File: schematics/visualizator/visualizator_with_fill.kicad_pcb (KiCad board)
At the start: 2 copper layers, 39.3 x 43.2 mm, 20 parts, among them J1 5V, J2 WS2812, J3 Audio, SW1 COLOR, SW2 PATTERN, U1 ATmega328-16PU, Y1 16MHz

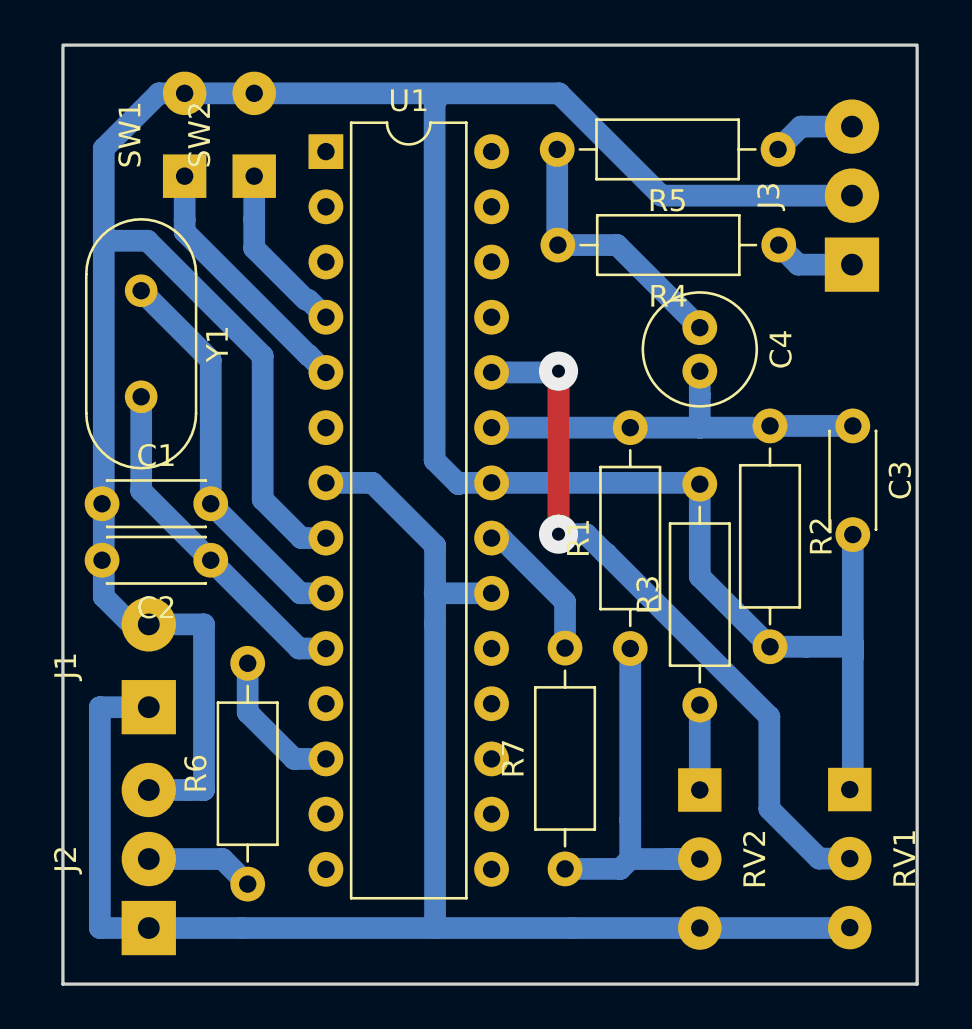
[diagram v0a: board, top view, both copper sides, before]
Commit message: PCBs updated
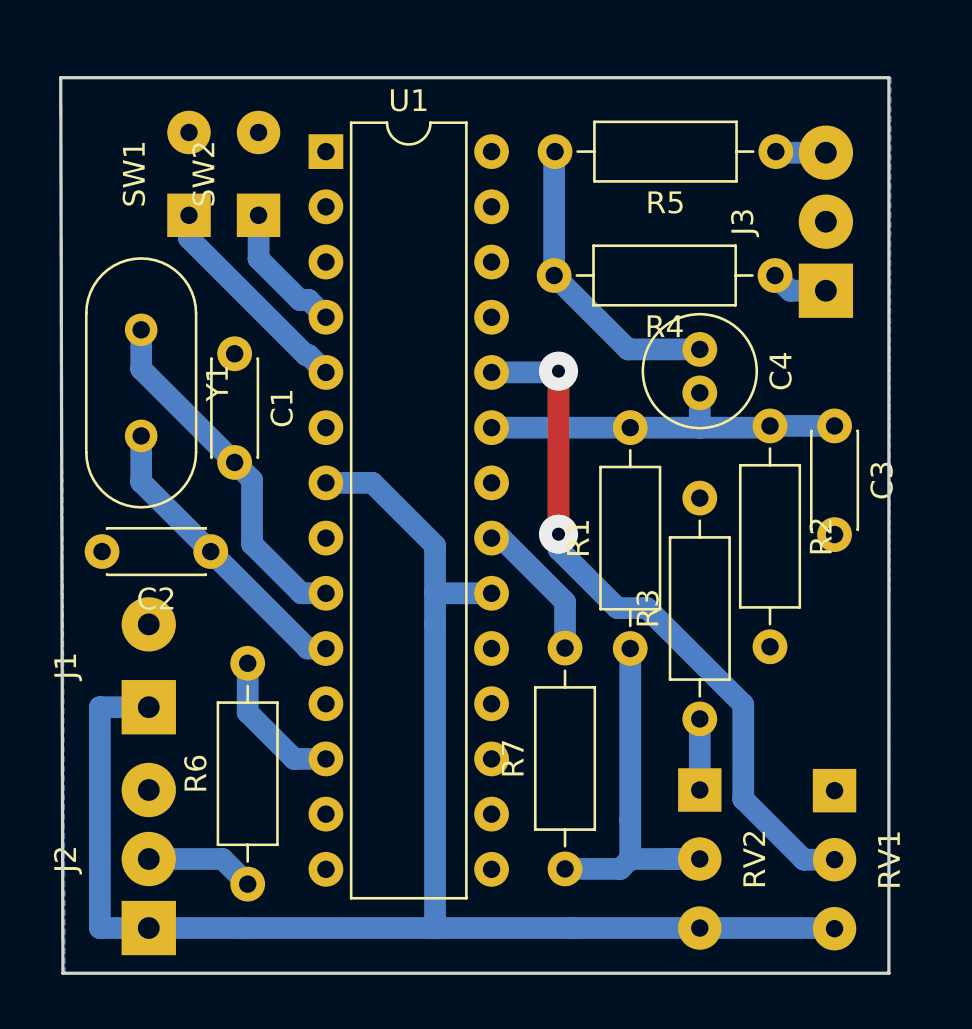
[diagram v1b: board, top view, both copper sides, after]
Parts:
- moved C1 9.21 mm to (61.9, 44.7), turned to 270 degrees
- moved SW2 1.81 mm to (63.0, 38.3)
- moved SW1 1.81 mm to (59.8, 38.3)
- moved Y1 1.80 mm to (57.6, 43.6)
- moved J3 1.70 mm to (89.1, 41.8)
- moved R4 1.41 mm to (86.8, 41.1)
- moved C4 1.00 mm to (83.3, 44.5)
- moved C3 0.84 mm to (89.5, 48.0)
- moved RV1 0.70 mm to (89.5, 64.8)
- moved R3 0.64 mm to (83.3, 61.5)
- moved C2 0.40 mm to (60.8, 53.8)
- moved R5 0.14 mm to (86.8, 35.4)
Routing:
- net Net-(C1-Pad1): track 146.7 -> 0.14 mm
- net Net-(C2-Pad1): track 15.8 -> 13.8 mm
- net Net-(C3-Pad1): track 19.3 -> 17.3 mm
- net Net-(C1-Pad2): track 18.1 -> 16.3 mm
- net Net-(SW1-Pad1): track 11.7 -> 9.91 mm
- net Net-(SW2-Pad1): track 7.81 -> 6.21 mm
- net Net-(J3-Pad3): track 3.83 -> 2.32 mm
- net Net-(C4-Pad1): track 12.5 -> 13.9 mm
- net Net-(J3-Pad1): track 3.74 -> 2.63 mm
- net Net-(J1-Pad1): track 74.2 -> 73.4 mm
- net Net-(R3-Pad1): track 3.91 -> 3.27 mm
- added copper zone on B.Cu, net Net-(C1-Pad1)
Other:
- board size 39.3 x 43.2 mm -> 38.1 x 41.2 mm
